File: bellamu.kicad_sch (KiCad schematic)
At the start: 19 parts, among them J1 Conn_Coaxial, J10 Conn_Coaxial, J2 Barrel_Jack_Switch_Pin3Ring, J3 Conn_Coaxial, J4 Conn_Coaxial, J5 472720001, J6 Conn_Coaxial, J8 Conn_Coaxial, P2 Header 2, P3 Header 2

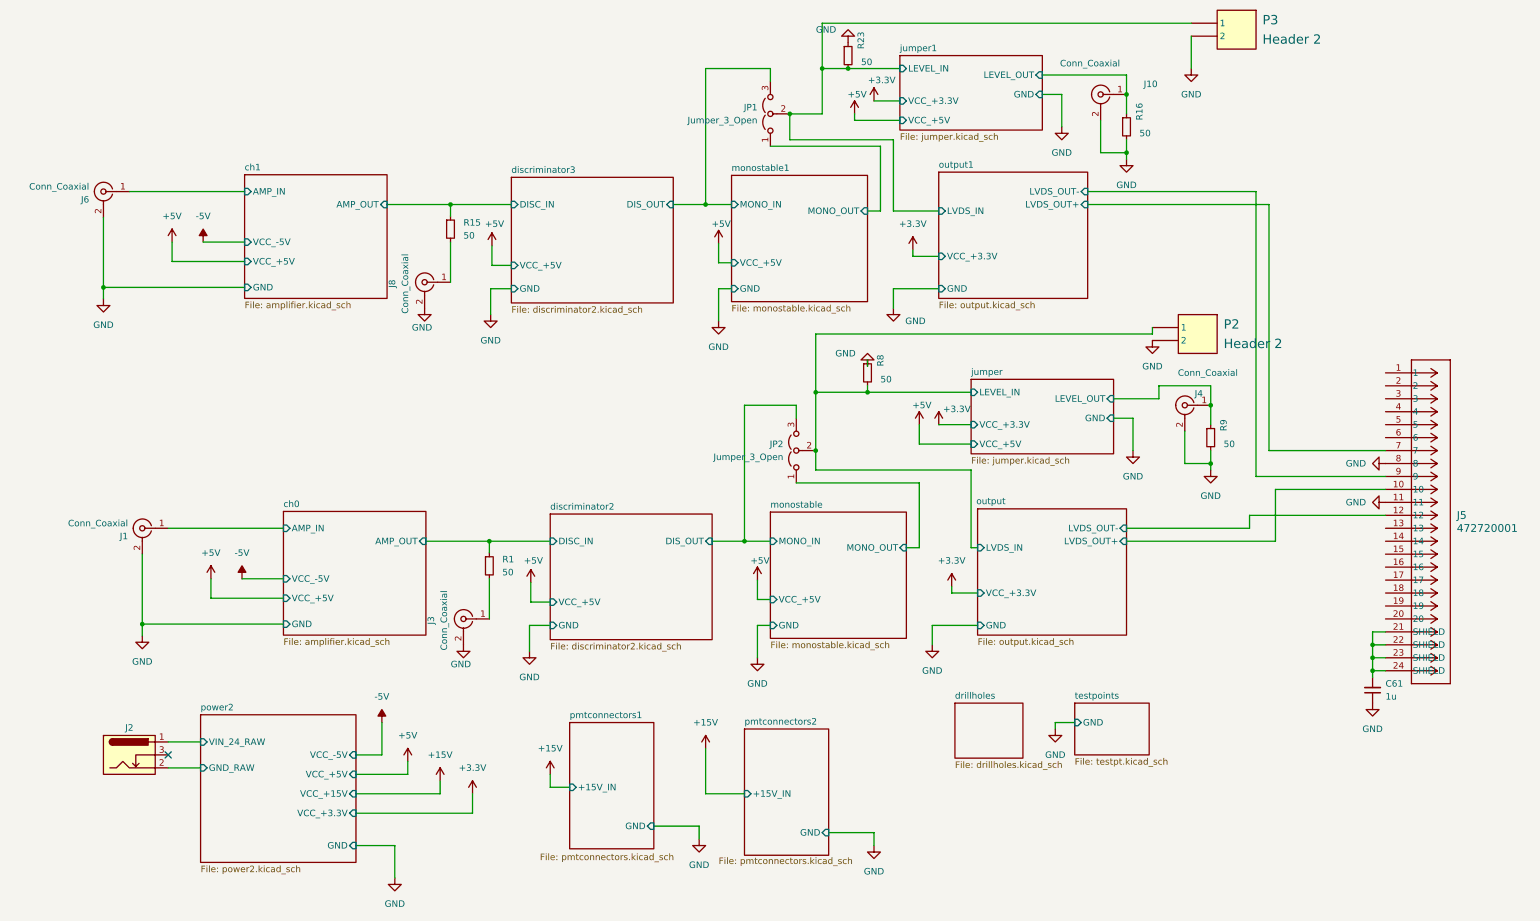
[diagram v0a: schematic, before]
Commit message: revised pcb and schematics
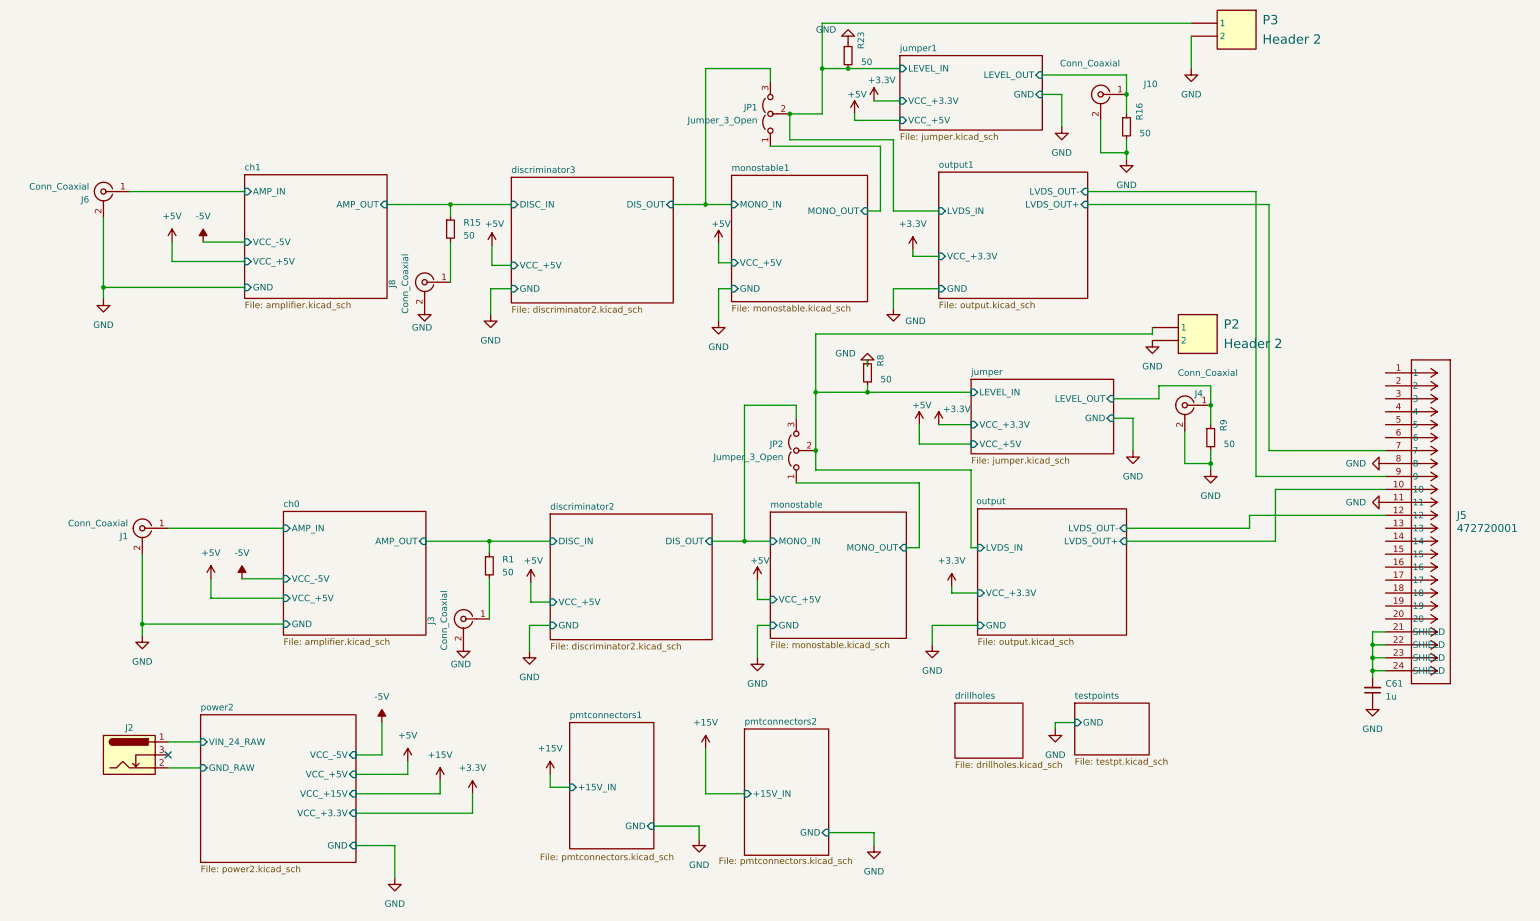
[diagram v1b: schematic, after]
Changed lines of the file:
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@@
 (kicad_sch
-	(version 20231120)
+	(version 20250114)
 	(generator "eeschema")
-	(generator_version "8.0")
+	(generator_version "9.0")
 	(paper "A4")
 	(junction
@@
 		(at 144.78 157.48)
 		(size 16.51 24.765)
+		(exclude_from_sim no)
+		(in_bom yes)
+		(on_board yes)
+		(dnp no)
 		(stroke
 			(width 0.1524)
@@
 		(at 186.055 152.4)
 		(size 13.335 10.795)
+		(exclude_from_sim no)
+		(in_bom yes)
+		(on_board yes)
+		(dnp no)
 		(fields_autoplaced yes)
 		(stroke
@@
 		(at 149.86 114.935)
 		(size 26.67 24.765)
+		(exclude_from_sim no)
+		(in_bom yes)
+		(on_board yes)
+		(dnp no)
 		(fields_autoplaced yes)
 		(stroke
@@
 		(at 99.06 49.276)
 		(size 31.75 24.638)
+		(exclude_from_sim no)
+		(in_bom yes)
+		(on_board yes)
+		(dnp no)
 		(fields_autoplaced yes)
 		(stroke
@@
 		(at 54.356 114.808)
 		(size 27.94 24.257)
+		(exclude_from_sim no)
+		(in_bom yes)
+		(on_board yes)
+		(dnp no)
 		(fields_autoplaced yes)
 		(stroke
@@
 		(at 190.5 114.3)
 		(size 29.21 24.765)
+		(exclude_from_sim no)
+		(in_bom yes)
+		(on_board yes)
+		(dnp no)
 		(stroke
 			(width 0.1524)
@@
 		(at 182.88 48.26)
 		(size 29.21 24.765)
+		(exclude_from_sim no)
+		(in_bom yes)
+		(on_board yes)
+		(dnp no)
 		(fields_autoplaced yes)
 		(stroke
@@
 		(at 106.68 115.316)
 		(size 31.75 24.638)
+		(exclude_from_sim no)
+		(in_bom yes)
+		(on_board yes)
+		(dnp no)
 		(fields_autoplaced yes)
 		(stroke
@@
 		(at 209.55 152.4)
 		(size 14.605 10.16)
+		(exclude_from_sim no)
+		(in_bom yes)
+		(on_board yes)
+		(dnp no)
 		(fields_autoplaced yes)
 		(stroke
@@
 		(at 110.49 156.21)
 		(size 16.51 24.765)
+		(exclude_from_sim no)
+		(in_bom yes)
+		(on_board yes)
+		(dnp no)
 		(stroke
 			(width 0.1524)
@@
 		(at 38.1 154.686)
 		(size 30.48 28.956)
+		(exclude_from_sim no)
+		(in_bom yes)
+		(on_board yes)
+		(dnp no)
 		(fields_autoplaced yes)
 		(stroke
@@
 		(at 142.24 48.895)
 		(size 26.67 24.765)
+		(exclude_from_sim no)
+		(in_bom yes)
+		(on_board yes)
+		(dnp no)
 		(fields_autoplaced yes)
 		(stroke
@@
 		(at 46.736 48.768)
 		(size 27.94 24.257)
+		(exclude_from_sim no)
+		(in_bom yes)
+		(on_board yes)
+		(dnp no)
 		(fields_autoplaced yes)
 		(stroke
@@
 		(at 175.26 25.4)
 		(size 27.94 14.605)
+		(exclude_from_sim no)
+		(in_bom yes)
+		(on_board yes)
+		(dnp no)
 		(fields_autoplaced yes)
 		(stroke
@@
 		(at 189.23 88.9)
 		(size 27.94 14.605)
+		(exclude_from_sim no)
+		(in_bom yes)
+		(on_board yes)
+		(dnp no)
 		(fields_autoplaced yes)
 		(stroke
@@
 		)
 	)
+	(embedded_fonts no)
 )
